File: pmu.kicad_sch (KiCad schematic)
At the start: 4 parts, among them SW1 Power ON SW, U2 MAX1555

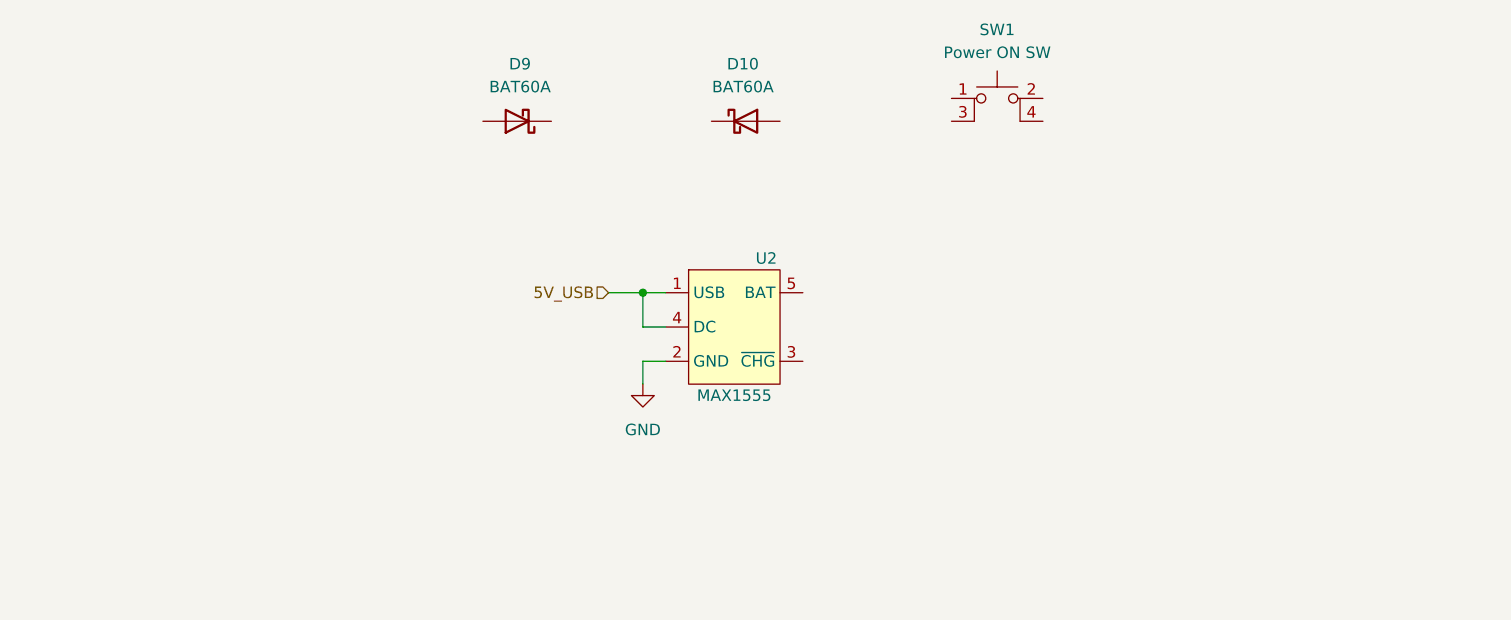
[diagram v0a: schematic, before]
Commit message: more stuff
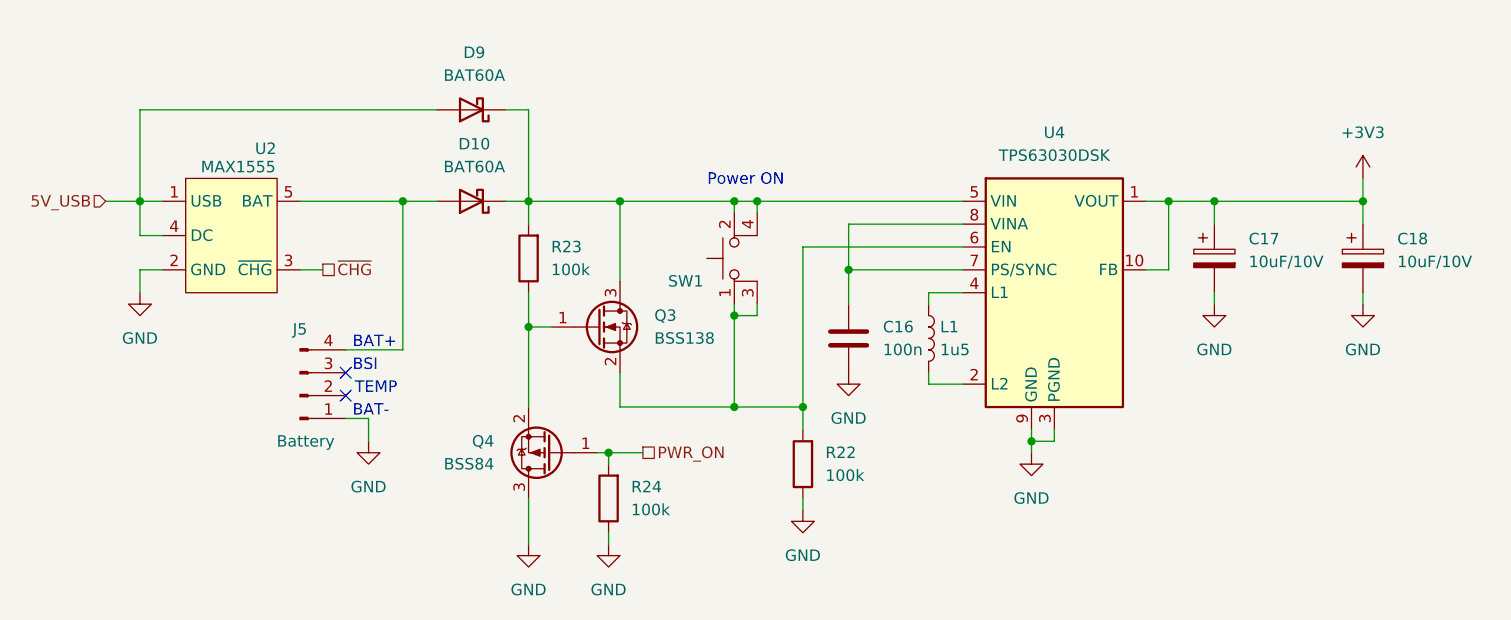
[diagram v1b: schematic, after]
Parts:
- added C16: 100n, Capacitor_SMD:C_0805_2012Metric, symbol Device:C
- added C17, C18: 10uF/10V, Capacitor_Tantalum_SMD:CP_EIA-3528-21_Kemet-B, symbol Device:C_Polarized
- added J5: Battery, symbol Connector:Conn_01x04_Pin
- added L1: 1u5, Inductor_SMD:L_1210_3225Metric, symbol Device:L
- added Q3: BSS138, Package_TO_SOT_SMD:SOT-23, symbol Transistor_FET:BSS138
- added Q4: BSS84, Package_TO_SOT_SMD:SOT-23, symbol Transistor_FET:BSS84
- added R22, R23, R24: 100k, Inductor_SMD:L_0805_2012Metric, symbol Device:R
- added U4: TPS63030DSK, Package_SON:WSON-10-1EP_2.5x2.5mm_P0.5mm_EP1.2x2mm, symbol Regulator_Switching:TPS63030DSK
- SW1: value Power ON SW -> ~
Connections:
- net 5V_USB: now also D9.2 (A)
- net GND: now also C16.1, C17.2, C18.2, J5.1 (Pin_1), Q4.3 (D), R22.1, R24.1, U4.11 (PGND), U4.3 (PGND), U4.9 (GND)
- net ~{CHG}: now reaches U2.3 (~{CHG})
- net at U2.5 (BAT): now also D10.2 (A), J5.4 (Pin_4)
- net at D9.1 (K): now also D10.1 (K), SW1.2, SW1.4 (A), Q3.3 (D), R23.2, U4.5 (VIN)
- net at SW1.1: now also SW1.3 (K), Q3.2 (S), R22.2, U4.6 (EN)
- new net: L1.2, U4.2 (L2)
- new net: L1.1, U4.4 (L1)
- new net: C16.2, U4.7 (PS/SYNC), U4.8 (VINA)
- new net: Q3.1 (G), Q4.2 (S), R23.1
- new net +3V3: C17.1, C18.1, U4.1 (VOUT), U4.10 (FB)
- new net PWR_ON: Q4.1 (G), R24.2
- no-connect marks 0 -> 2
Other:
- note added: "BAT+"
- note added: "BAT-"
- note added: "BSI"
- note added: "Power ON"
- note added: "TEMP"
- moved on the sheet: D10, D9, SW1, U2
